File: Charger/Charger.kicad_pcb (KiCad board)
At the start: 2 copper layers, 156 parts, among them J1 Bat_ballanser_conn, J2 Battery_conn, J3 Power_conn, Q1 BC846BW, Q10 MJD45H11T4, Q11 MJD45H11T4, Q12 MJD45H11T4, Q13 BC846BW, Q14 MJD31CT4, Q15 BUJ302AD, Q16 BUJ302AD, Q17 IRF7404, Q18 IRF7404, Q19 BC846BW, Q2 BC846BW, Q3 BC846BW, Q4 MJD45H11T4, Q5 MJD45H11T4, Q6 MJD45H11T4, Q7 BC846BW, Q8 BC846BW, Q9 BC846BW, U1 LM2904, U10 MCP6001-OT, U11 MCP6001-OT, U12 ACS712xLCTR-20A, U13 MCP6001-OT, U14 MCP6001-OT, U15 MCP6001-OT, U16 MCP6001-OT, U17 XL4015, U18 XL4015, U19 MCP6001-OT, U2 LM2904, U20 LM2575-12BU, U21 L7805, U22 LDI1117-3.3, U23 RaspberryPi_Pico, U3 LM2904, U4 LM2904, U5 LM2904, U6 LM2904, U7 MCP6001-OT, U8 MCP6001-OT, U9 MCP6001-OT

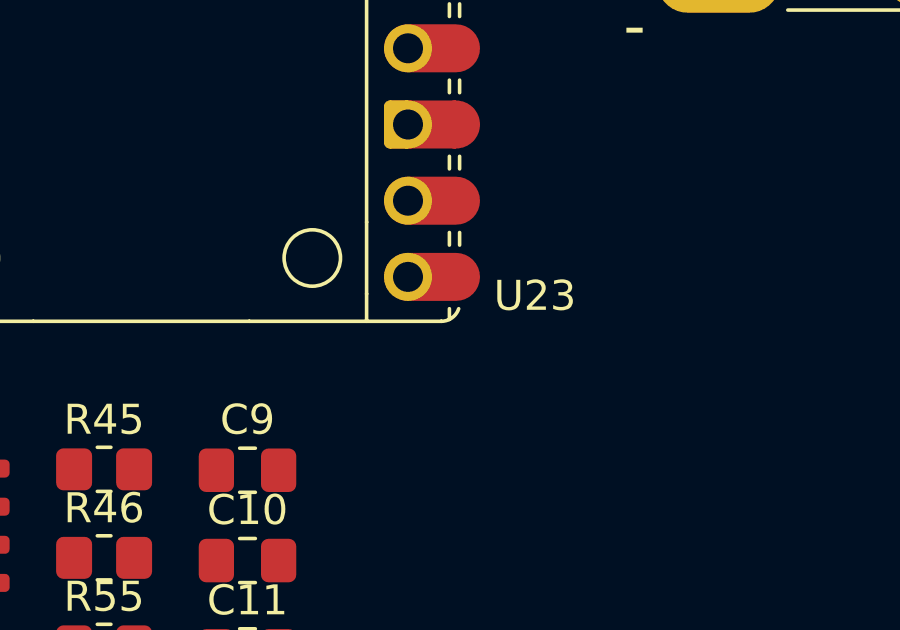
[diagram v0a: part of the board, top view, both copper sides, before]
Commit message: UPDATE UC
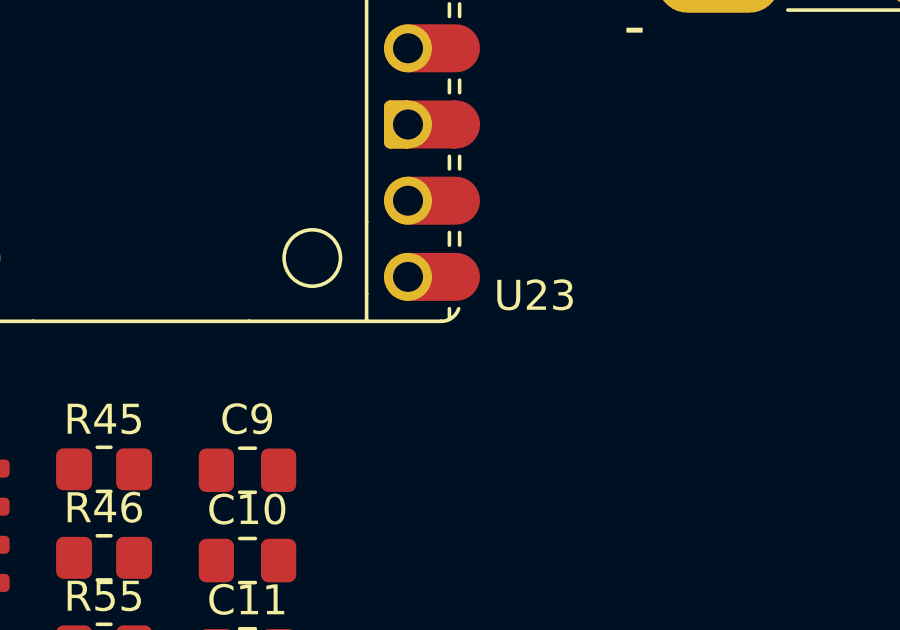
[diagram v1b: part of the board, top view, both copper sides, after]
